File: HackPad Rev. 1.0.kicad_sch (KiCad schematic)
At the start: 14 parts, among them SW1 SW_Push_45deg, SW2 SW_Push_45deg, SW3 SW_Push_45deg, SW4 SW_Push_45deg, SW5 RotaryEncoder_Switch, SW6 SW_Push_45deg, U1 Seeed Studio XIAO SAMD21

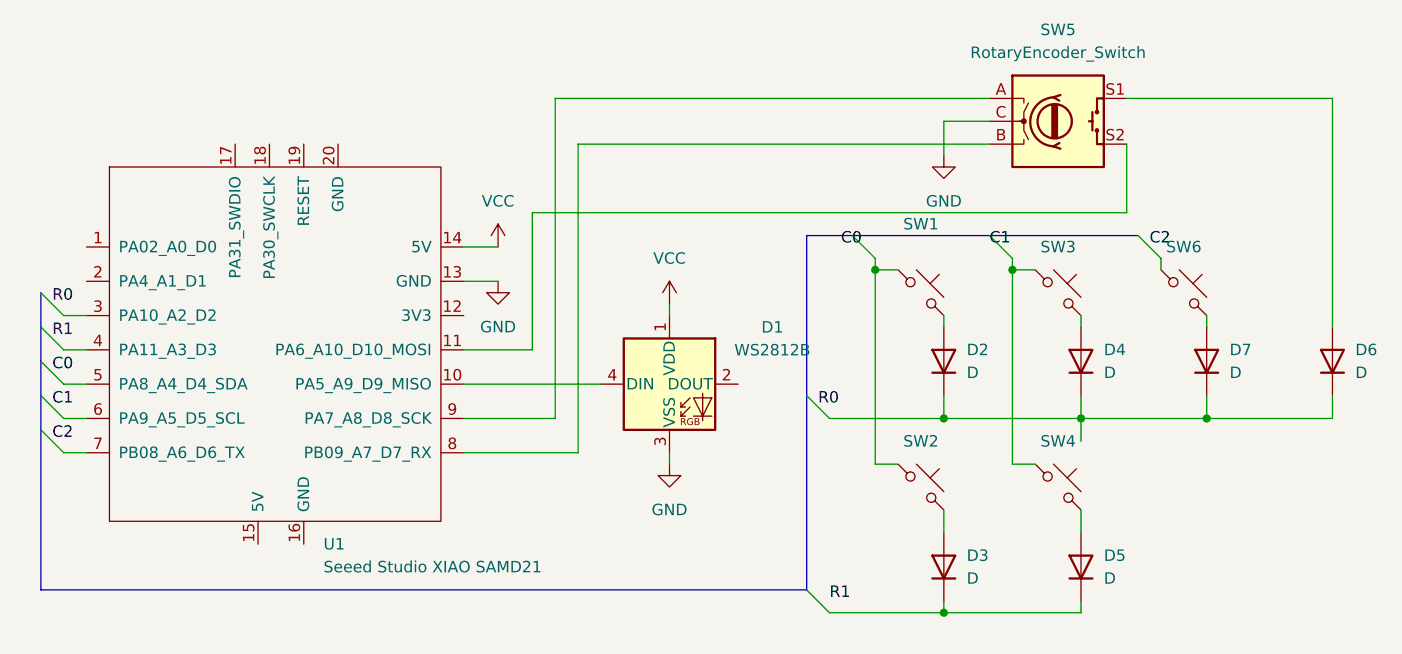
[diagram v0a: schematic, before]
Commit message: finished PCB
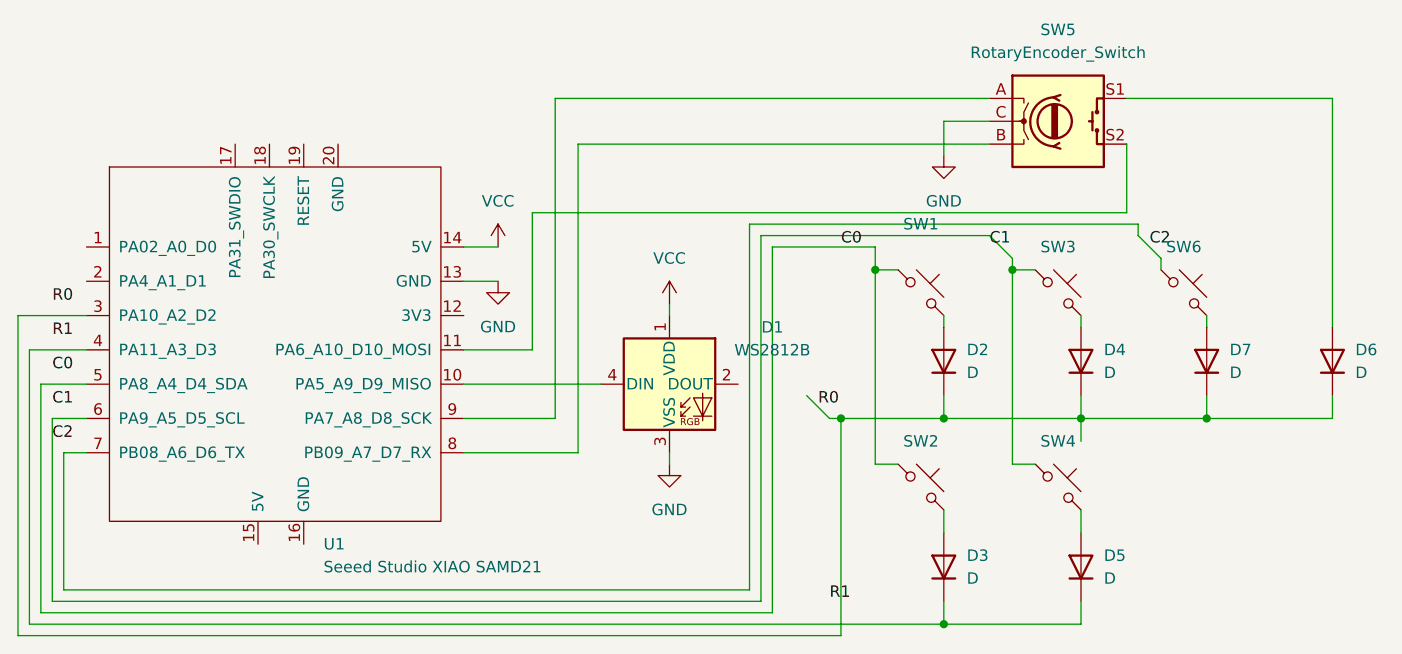
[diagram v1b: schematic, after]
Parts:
- SW1, SW2, SW3, SW4: footprint MX_Solderable:MX-Solderable-1U -> Button_Switch_Keyboard:SW_Cherry_MX_1.00u_PCB
- SW5: footprint (none) -> Rotary_Encoder:RotaryEncoder_Alps_EC11E-Switch_Vertical_H20mm
- SW6: footprint MX_Solderable:MX-Solderable-1U -> Button_Switch_Keyboard:SW_Cherry_MX_2.00u_PCB
- U1: footprint (none) -> footprints:XIAO-Generic-Thruhole-14P-2.54-21X17.8MM
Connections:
- net C0: now also SW1.1, SW2.1, U1.5 (PA8_A4_D4_SDA)
- net C2: now also U1.6 (PA9_A5_D5_SCL)
- net at D3.1 (K), D5.1 (K): now also U1.4 (PA11_A3_D3)
- net at D2.1 (K), D4.1 (K), D6.1 (K)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: now also U1.3 (PA10_A2_D2)
